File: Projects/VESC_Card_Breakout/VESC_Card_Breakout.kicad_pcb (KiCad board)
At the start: 2 copper layers, 9 parts, among them P1 USB_OTG, P2 CONN_01X02, P3 CONN_01X04, P4 EC90_Flat, P5 CONN_01X02, P6 AMP17614426-2_EDGE, P7 CONN_01X06

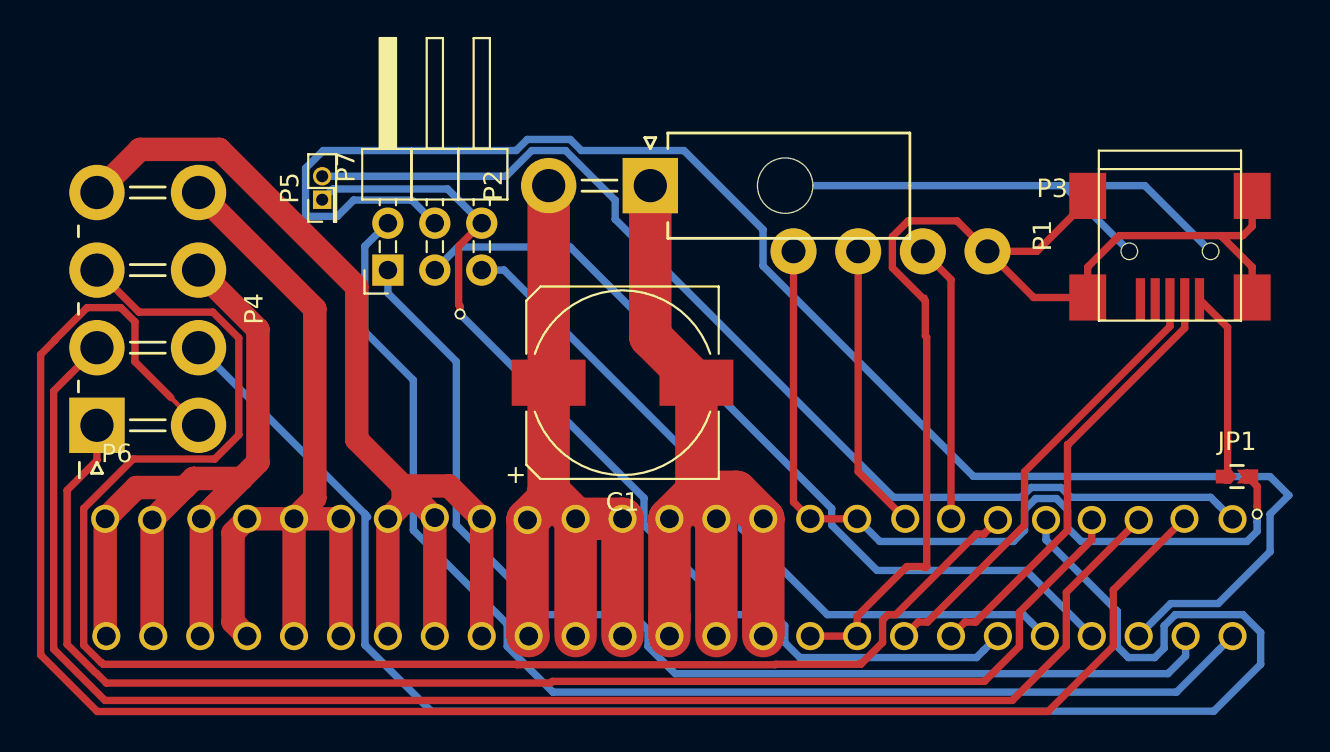
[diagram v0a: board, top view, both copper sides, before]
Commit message: Rotated component
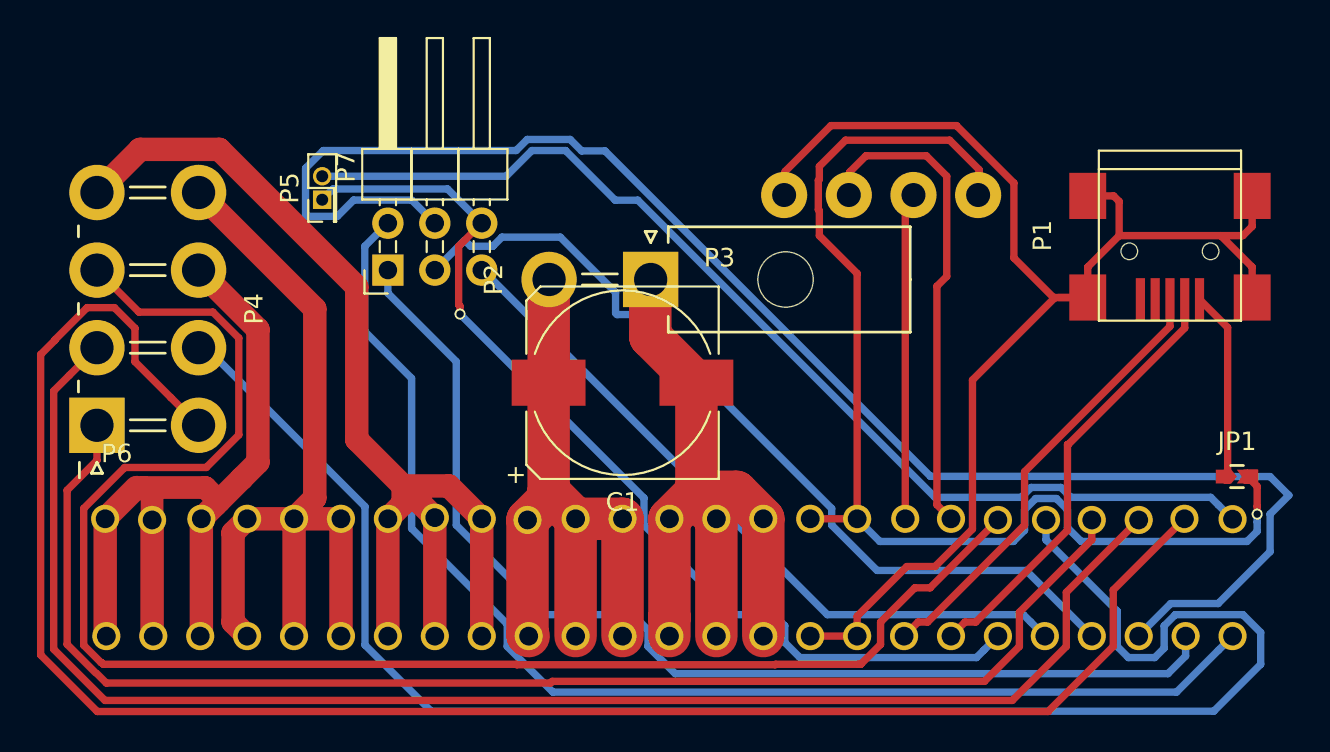
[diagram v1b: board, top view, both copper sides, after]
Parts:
- moved P3 10.4 mm to (178.8, 43.2), turned to 180 degrees
- moved P2 5.08 mm to (161.0, 47.8)
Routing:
- net (no net): track 29.5 -> 0.00 mm
- net /5v0: track 46.1 -> 62.0 mm
- net /Motor_Controller/CANL/RX: track 15.1 -> 25.9 mm
- net /Motor_Controller/PGND: track 44.9 -> 39.6 mm
- net /Motor_Controller/VBAT: track 42.2 -> 37.2 mm
- net /GNDD: track 72.0 -> 77.0 mm
- net /Motor_Controller/CANH/TX: track 15.5 -> 18.2 mm
- net /Motor_Controller/W: track 46.6 -> 44.2 mm
- net Net-(P6-Pad19): track 45.3 -> 46.7 mm
- net Net-(P6-Pad18): track 85.9 -> 84.8 mm
- net Net-(P5-Pad2): track 59.2 -> 58.6 mm
